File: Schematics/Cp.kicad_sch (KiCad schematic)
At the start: 42 parts, among them Q10 2SK30A, Q11 2SK30A, Q5 2SC1815, Q6 2SC1815, Q7 2SC1815, Q8 2SC1815, SW1 SW_DPDT_x2, U3 CA3080

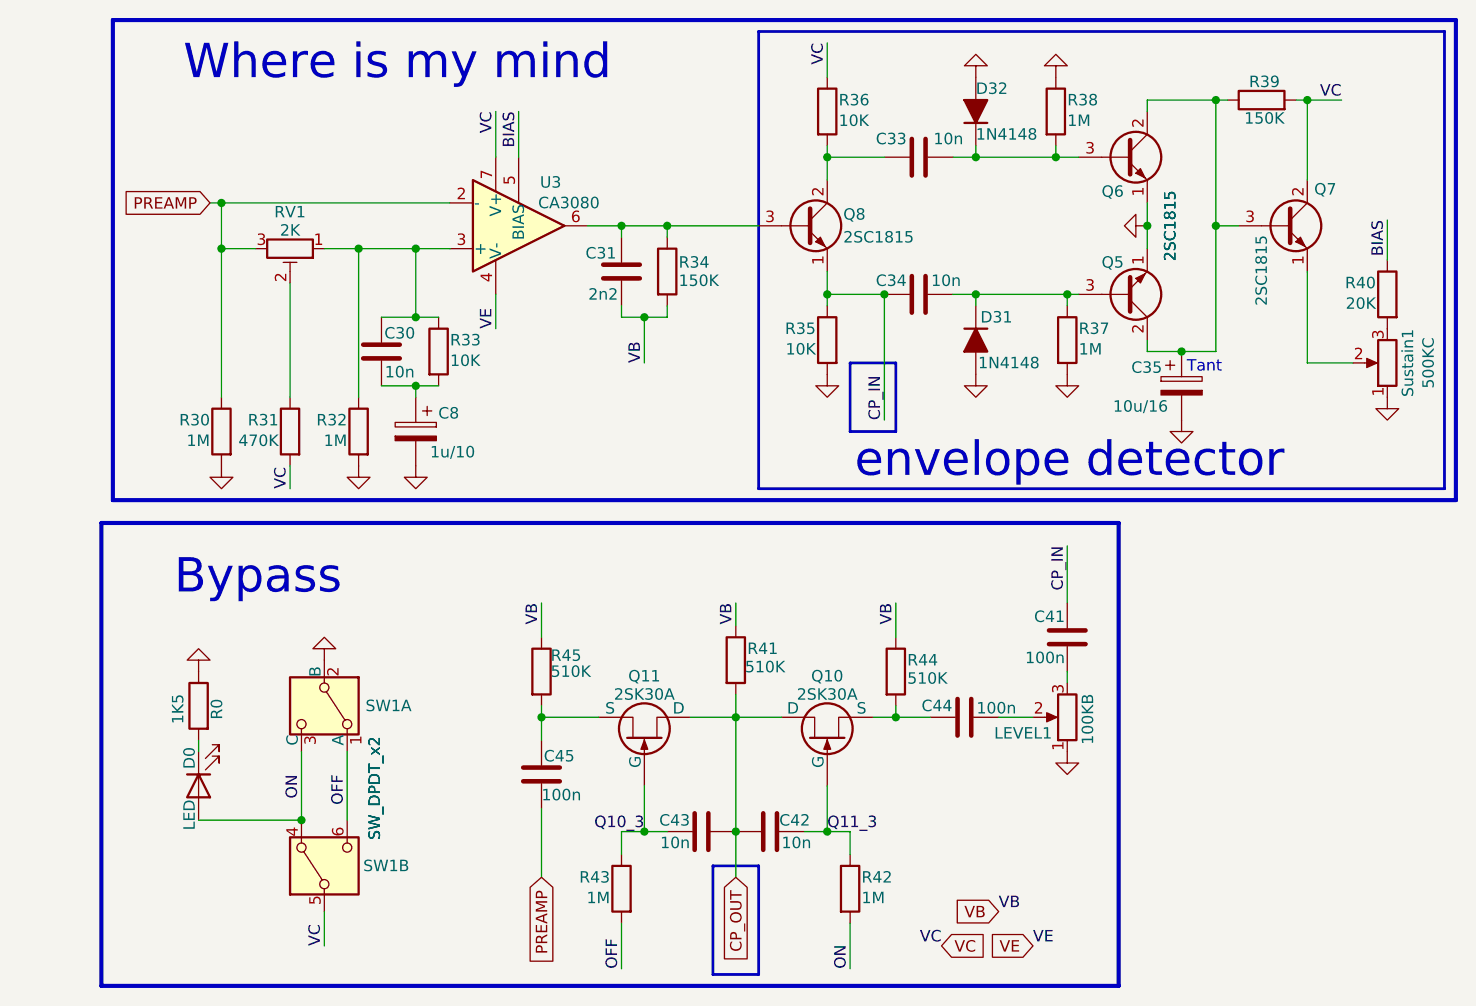
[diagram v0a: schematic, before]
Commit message: Cosmetic upd
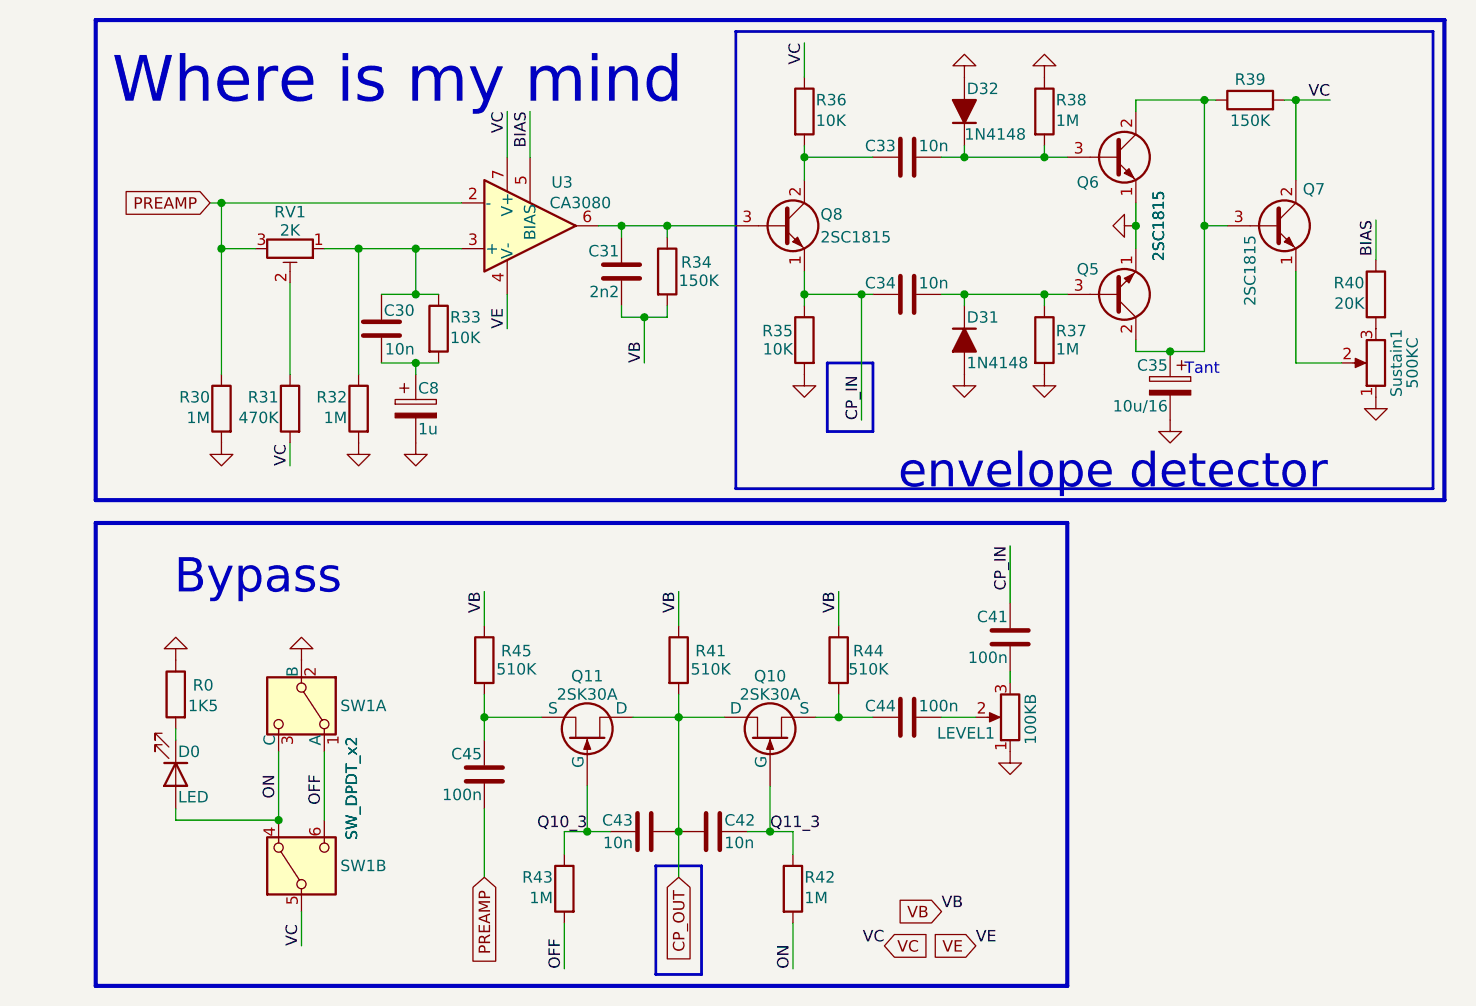
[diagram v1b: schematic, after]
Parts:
- C8: value 1u/10 -> 1u
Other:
- moved on the sheet: C30, C33, C34, C35, C41, C42, C43, C44, C45, C8, D0, D31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
